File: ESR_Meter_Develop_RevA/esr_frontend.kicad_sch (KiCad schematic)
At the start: 46 parts, among them K1 1462038-4, U1 TL074HIDR, U2 TL074HIDR

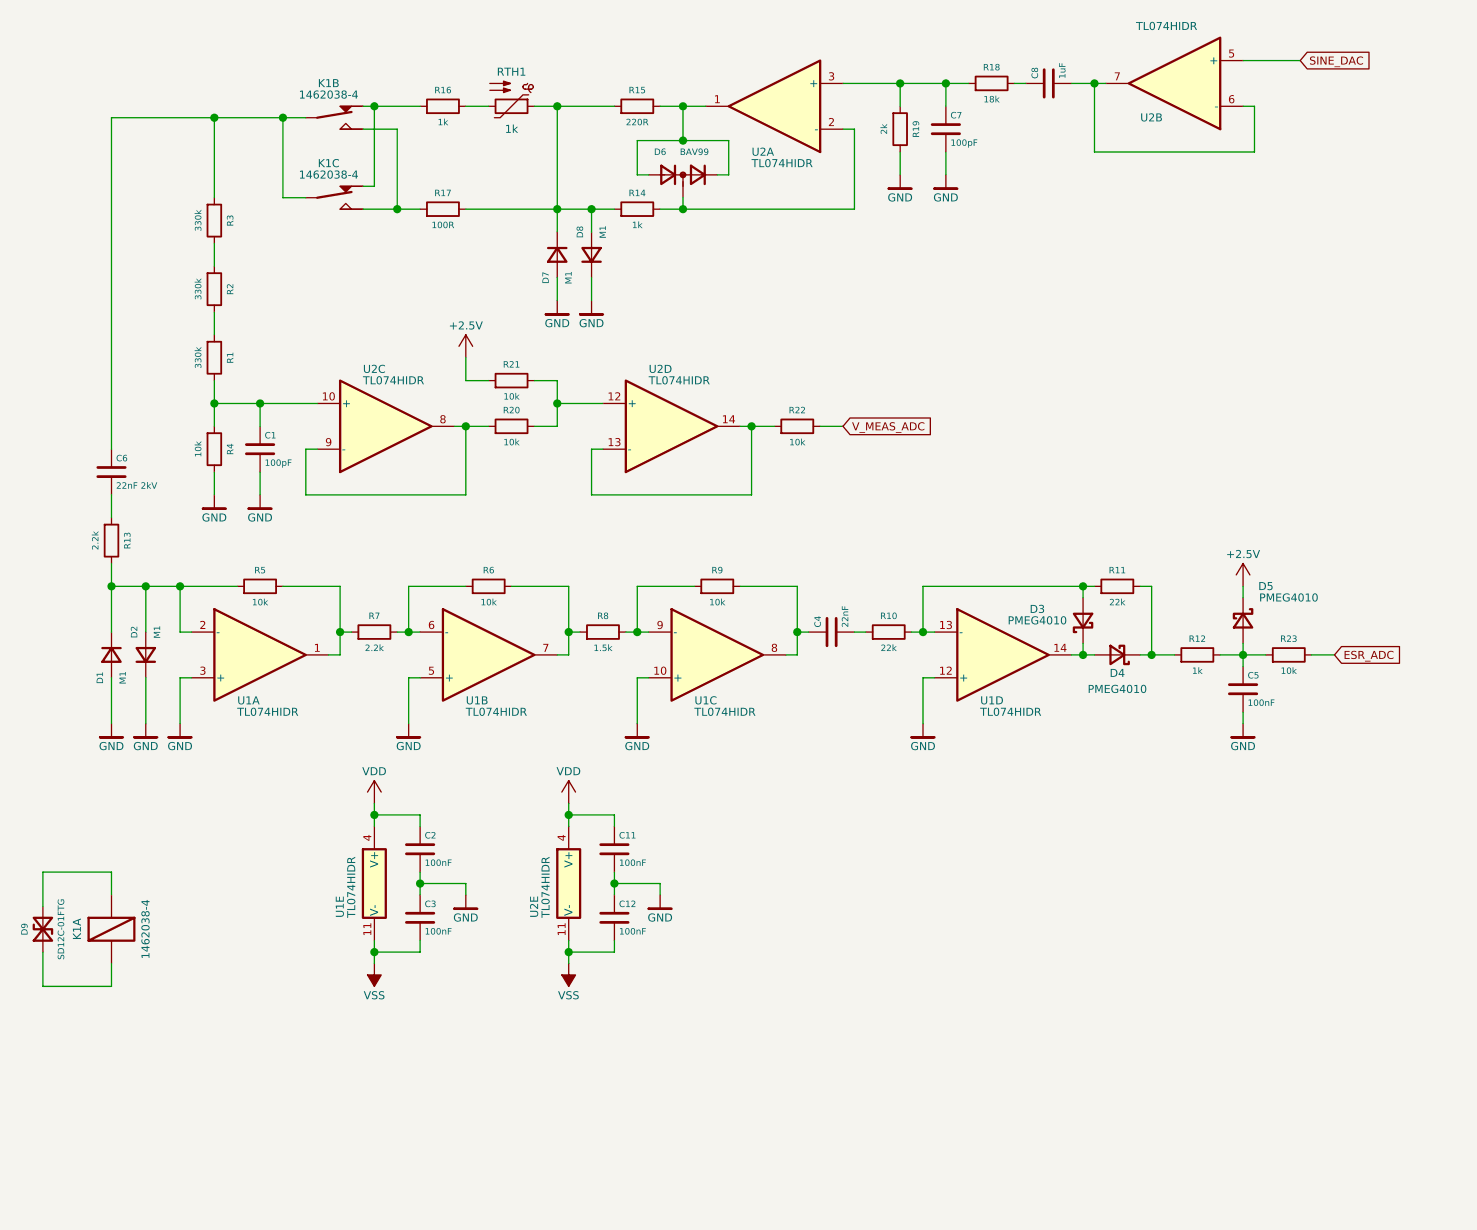
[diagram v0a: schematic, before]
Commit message: backup WIP
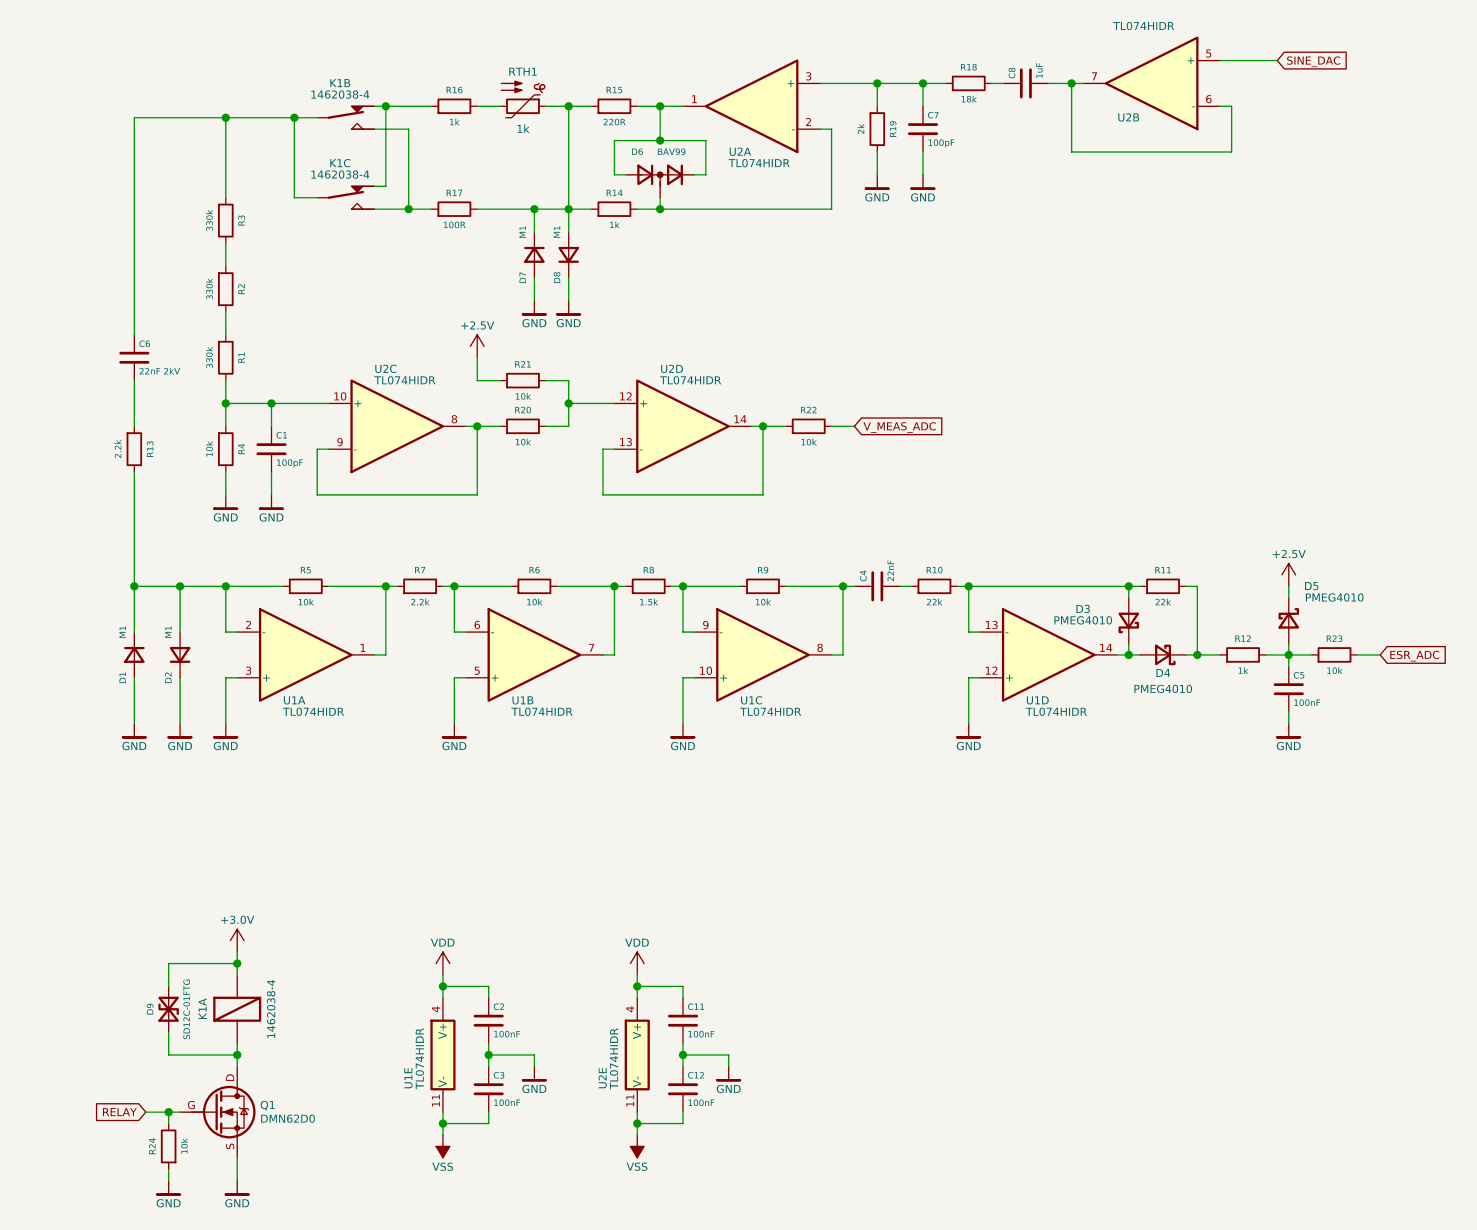
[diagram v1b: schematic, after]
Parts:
- added Q1: DMN62D0, 3Brain_Transistors:SOT-23_GSD, symbol 3Brain_Transistors:DMN62D0U-7
- added R24: 10k, 3Brain_Resistors:R_0603, symbol 3Brain_Resistors:K_10k_0603
- added unit 3 of U2
- added unit 4 of U2
- added unit 1 of U2
- added unit 2 of U2
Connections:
- net GND: now also Q1.S, R24.1
- net SINE_DAC: now also U2.5 (+); no longer U2.5 (+)
- net at C7.1, R18.1, R19.1: now also U2.3 (+); no longer U2.3 (+)
- net at D9.A1, K1.8: now also Q1.D
- net +3.0V: now reaches D9.A2, K1.1 (+)
- net at C1.1, R1.2, R4.1: now also U2.10 (+); no longer U2.10 (+)
- net at D6.A, D6.C, R15.2: now also U2.1; no longer U2.1
- net at R20.2, R21.2: now also U2.12 (+); no longer U2.12 (+)
- net at D6.AC, R14.2: now also U2.2 (-); no longer U2.2 (-)
- new net: R20.1, U2.8, U2.9 (-)
- new net: R22.1, U2.13 (-), U2.14
- new net: C8.2, U2.6 (-), U2.7
- new net RELAY: Q1.G, R24.2
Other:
- moved on the sheet: C1, C11, C12, C2, C3, C4, C5, C6, C7, C8, D1, D2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
